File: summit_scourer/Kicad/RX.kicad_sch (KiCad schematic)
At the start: 11 parts, among them J3 Conn_Coaxial, Q2 2N7002H, U1 SI4732-A10-GS, Y1 32.768 KHz

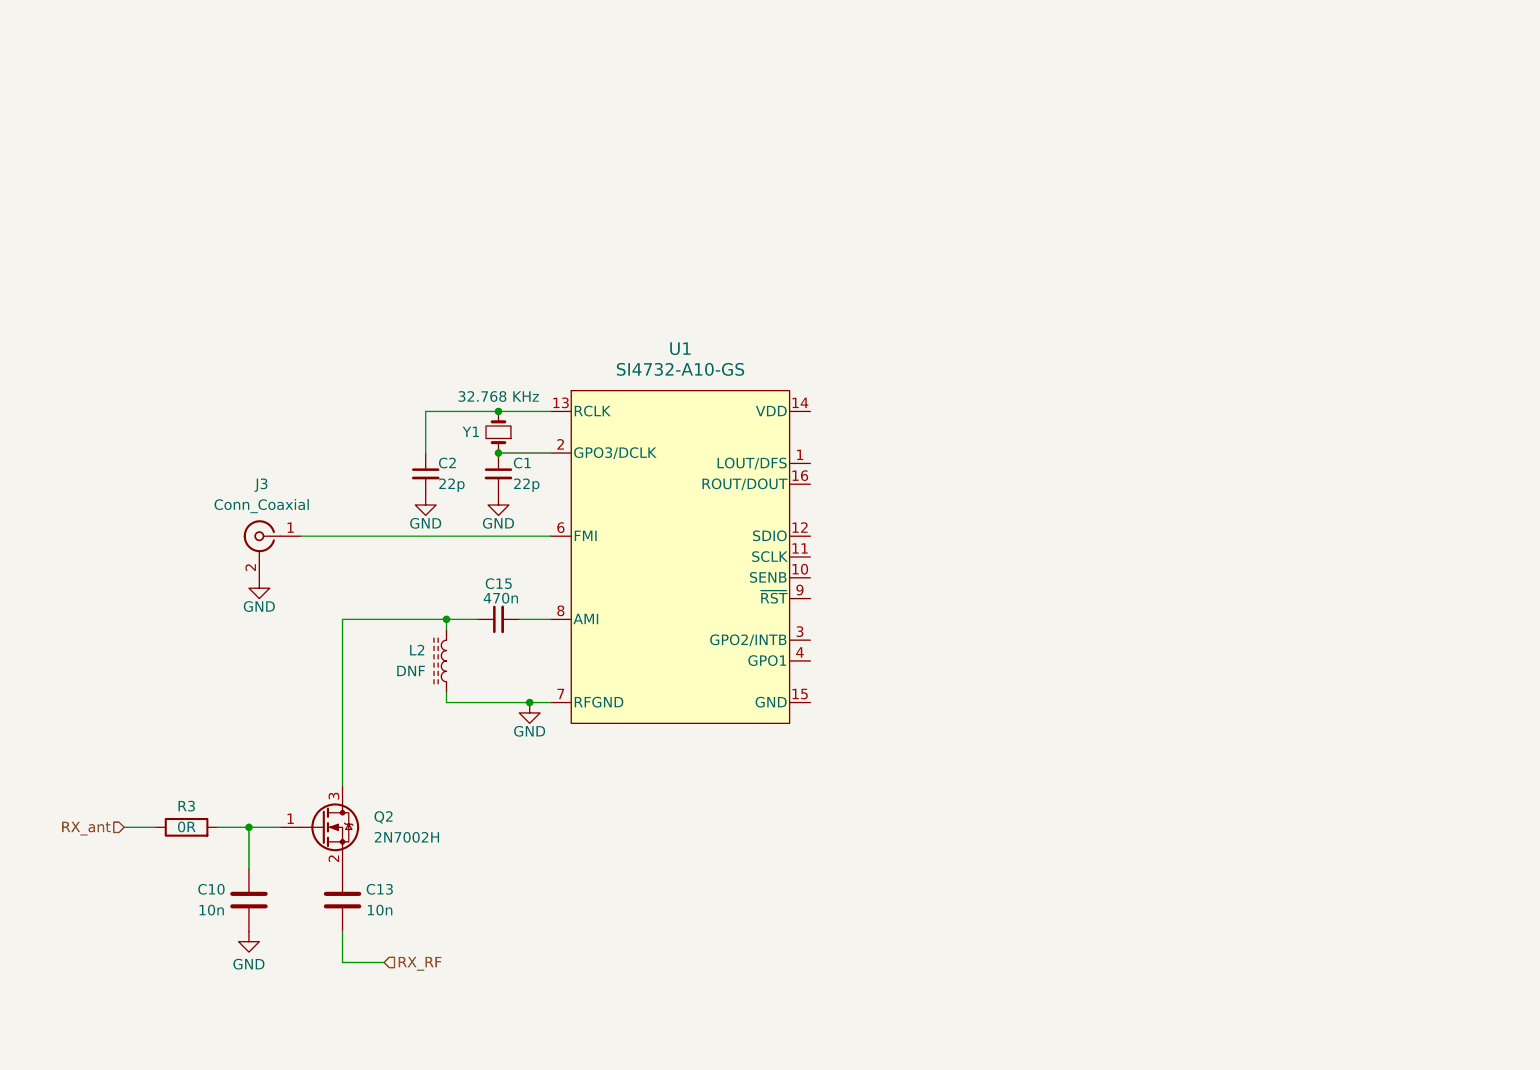
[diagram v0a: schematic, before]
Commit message: Add files via upload
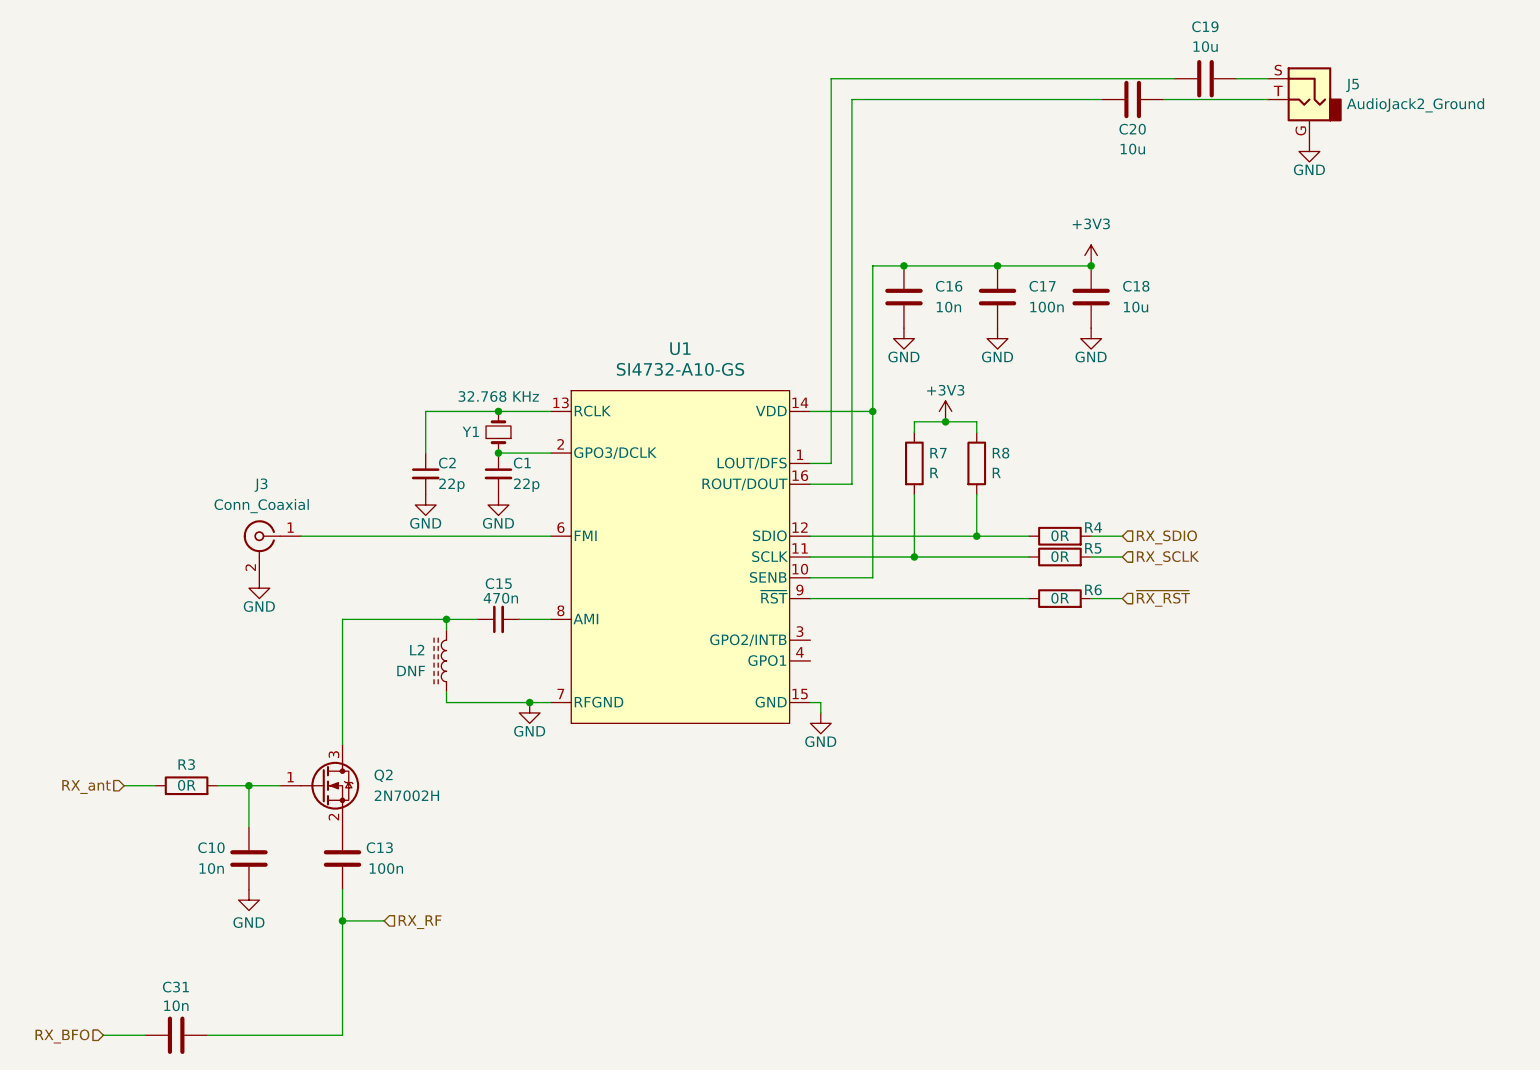
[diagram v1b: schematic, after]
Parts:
- added C16, C31: 10n, Capacitor_SMD:C_0603_1608Metric_Pad1.08x0.95mm_HandSolder, symbol Device:C
- added C17: 100n, Capacitor_SMD:C_0504_1310Metric_Pad0.83x1.28mm_HandSolder, symbol Device:C
- added C18, C19, C20: 10u, Capacitor_SMD:C_1210_3225Metric_Pad1.33x2.70mm_HandSolder, symbol Device:C
- added J5: AudioJack2_Ground, symbol Connector_Audio:AudioJack2_Ground
- added R4, R5, R6: 0R, symbol Device:R
- added R7, R8: R, symbol Device:R
- C13: value 10n -> 100n
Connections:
- net GND: now also U1.15 (GND), C16.2, C17.2, C18.2, J5.G
- net RX_RF: now also C31.1
- net at U1.1 (LOUT/DFS): now also C19.1
- net +3V3: now reaches U1.10 (SENB)
- net +3V3: now also U1.14 (VDD), C16.1, C17.1, C18.1, R7.1, R8.1
- net at U1.11 (SCLK): now also R5.1, R7.2
- net at U1.12 (SDIO): now also R4.1, R8.2
- net at U1.16 (ROUT/DOUT): now also C20.1
- net at U1.9 (~{RST}): now also R6.1
- new net: C19.2, J5.S
- new net: C20.2, J5.T
- new net RX_BFO: C31.2
- new net RX_SCLK: R5.2
- new net RX_SDIO: R4.2
- new net ~{RX_RST}: R6.2
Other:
- moved on the sheet: C10, C13, Q2, R3

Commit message: Add files via upload
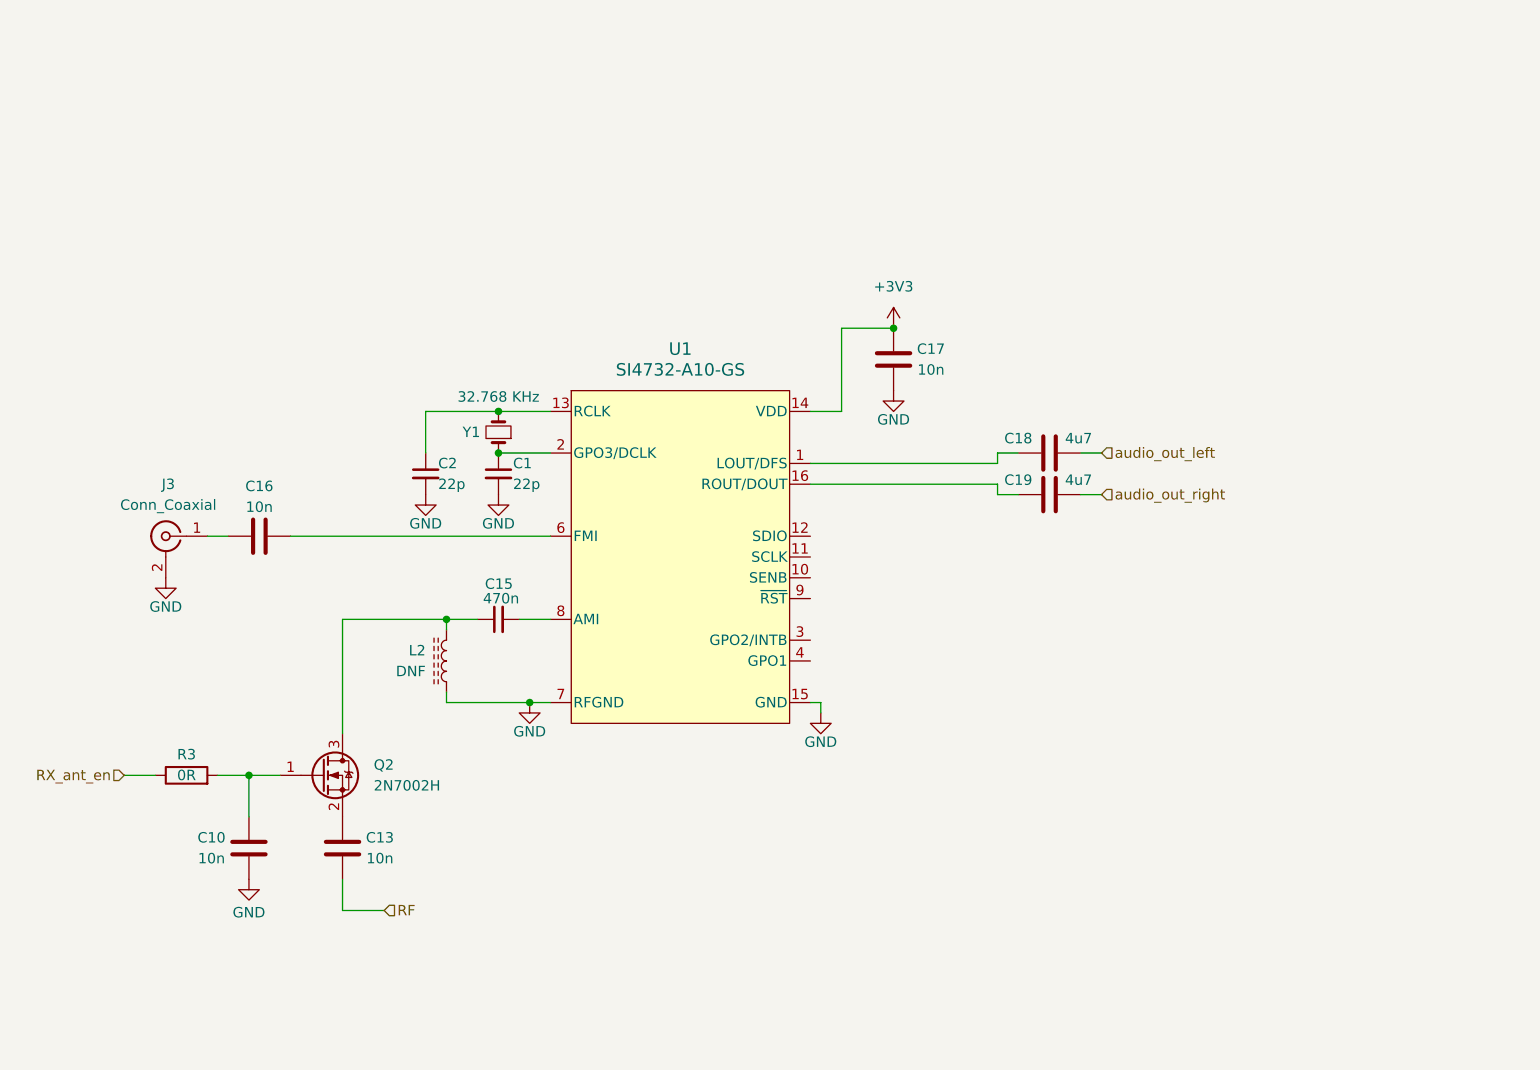
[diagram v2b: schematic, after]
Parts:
- removed C20: 10u, Capacitor_SMD:C_1210_3225Metric_Pad1.33x2.70mm_HandSolder, symbol Device:C
- removed C31: 10n, Capacitor_SMD:C_0603_1608Metric_Pad1.08x0.95mm_HandSolder, symbol Device:C
- removed J5: AudioJack2_Ground, symbol Connector_Audio:AudioJack2_Ground
- removed R4, R5, R6: 0R, symbol Device:R
- removed R7, R8: R, symbol Device:R
- C13: value 100n -> 10n
- C17: value 100n -> 10n; footprint Capacitor_SMD:C_0504_1310Metric_Pad0.83x1.28mm_HandSolder -> Capacitor_SMD:C_0603_1608Metric_Pad1.08x0.95mm_HandSolder
- C18, C19: value 10u -> 4u7; footprint Capacitor_SMD:C_1210_3225Metric_Pad1.33x2.70mm_HandSolder -> Capacitor_SMD:C_0603_1608Metric
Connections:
- net +3V3: no longer C16.1, C18.1, U1.10 (SENB)
- net GND: no longer C16.2, C18.2
- net at J3.1 (In): now also C16.1; no longer U1.6 (FMI)
- net audio_out_right: now reaches C19.2
- net at U1.16 (ROUT/DOUT): now also C19.1
- net at U1.1 (LOUT/DFS): now also C18.1; no longer C19.1
- net RX_RF renamed RF
- net RX_ant renamed RX_ant_en
- new net: C16.2, U1.6 (FMI)
- new net audio_out_left: C18.2
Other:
- moved on the sheet: C10, C13, J3, Q2, R3
